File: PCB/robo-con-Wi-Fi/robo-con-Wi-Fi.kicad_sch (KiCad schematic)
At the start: 118 parts, among them J1 Conn_01x04, J2 SMA-J, J3 Conn_01x05, J4 Conn_01x01, J5 Conn_01x02, J6 Conn_01x01, J7 Conn_01x06, Q1 2SC3325-Y, SW1 SW_Push, SW2 SW_Push, U1 STM32H723VGTx, U10 MCP73831-2-OT, U11 LM66100DCK, U12 NJM12877, U13 TXB0606DYYR, U14 TPS628513DRLR, U15 LM66100DCK, U18 USB_Type-C, U2 LBEE5HY2FY, U3 TXU0204, U5 RKJXV122400R, U6 IS25LP064D-JLLE, U7 RKJXV122400R, U8 TMHU28, U9 TMHU28, Y2 XRCGB25M000FFS1AR0

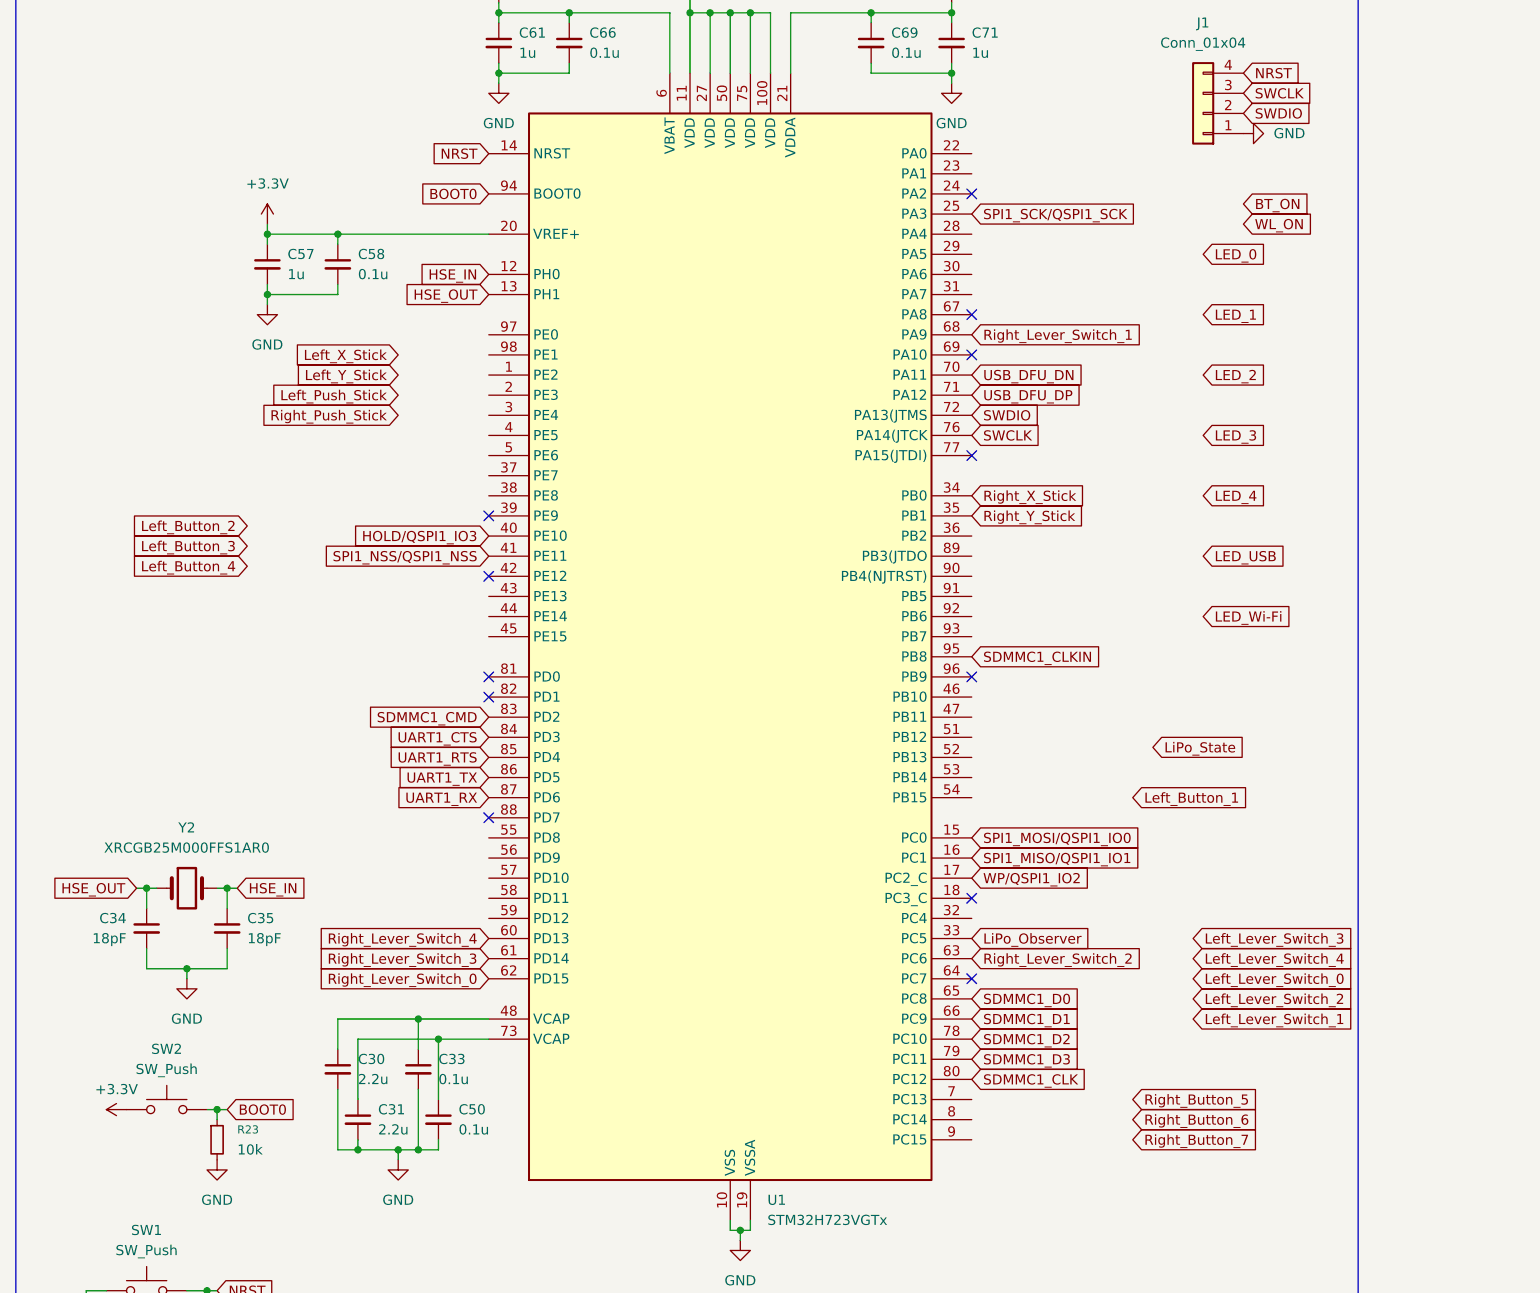
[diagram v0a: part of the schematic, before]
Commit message: PCB配線した　長さ合わせた後確認
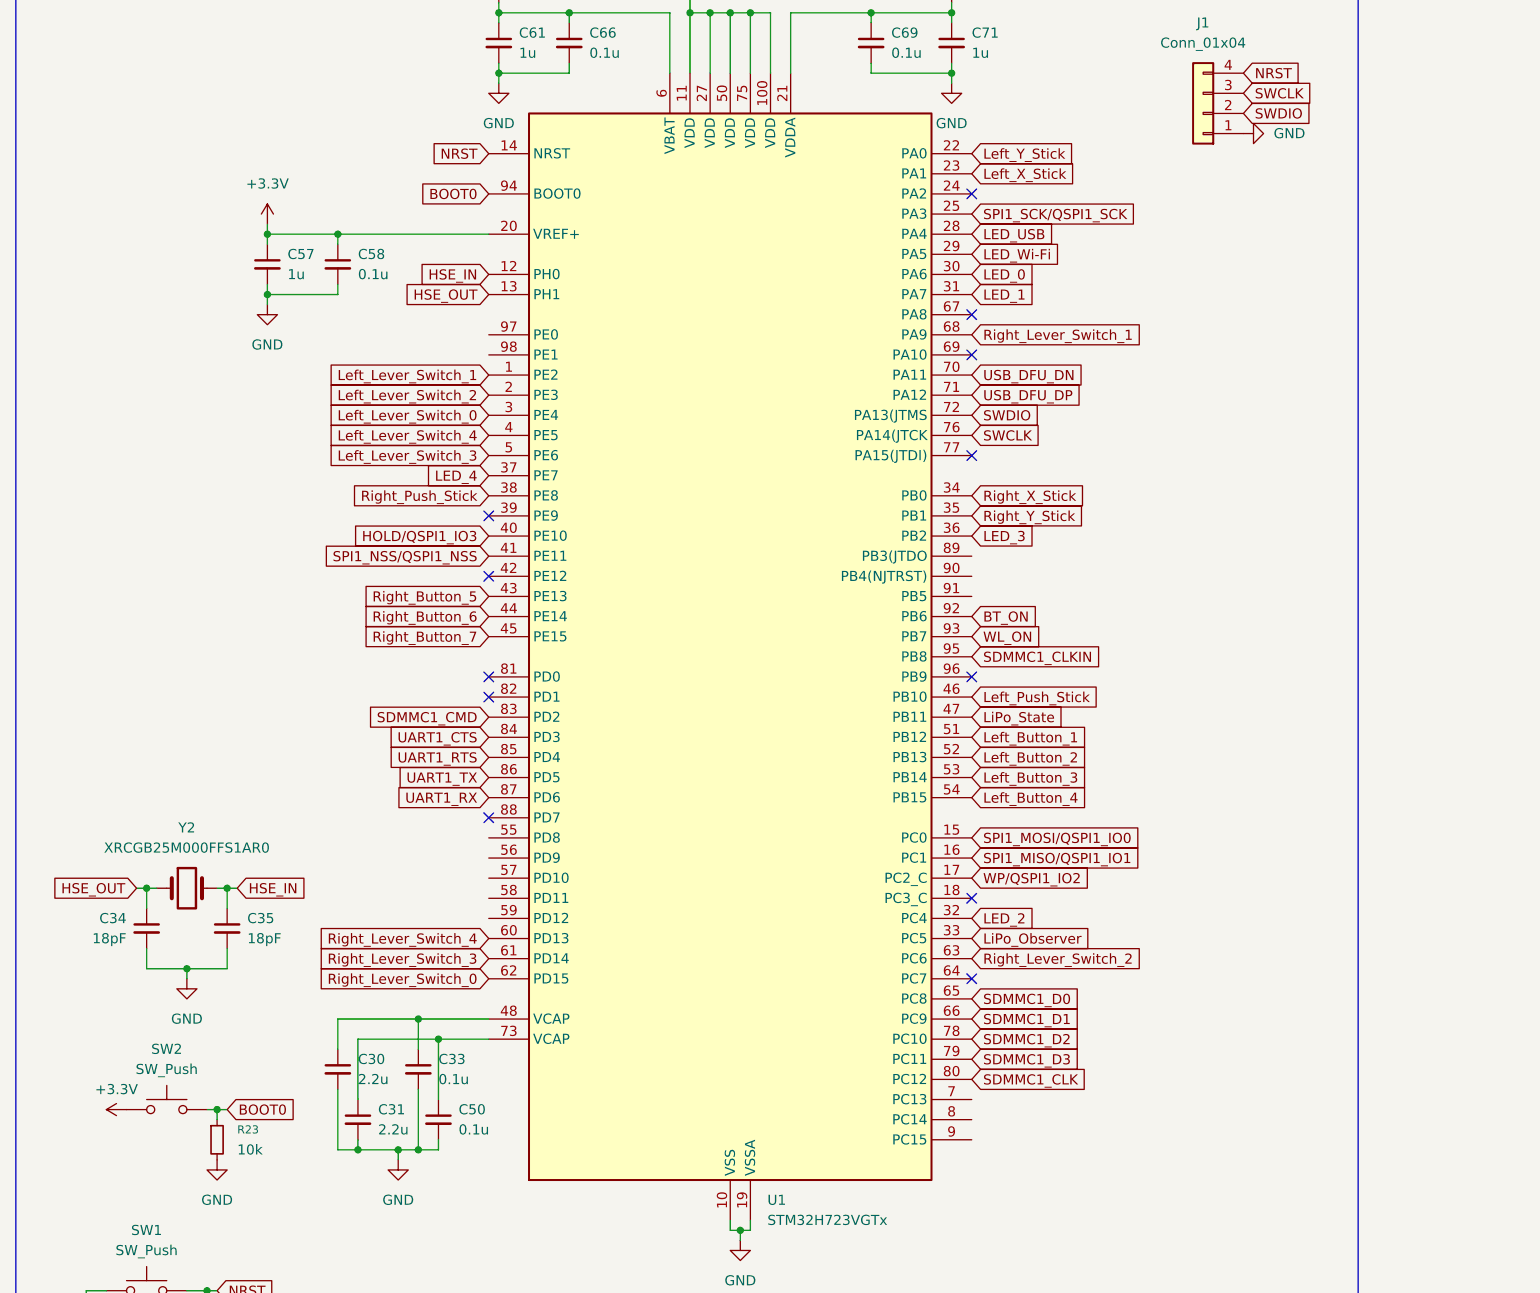
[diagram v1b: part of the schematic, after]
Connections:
- net BT_ON: now also U1.92 (PB6)
- net LED_0: now also U1.30 (PA6)
- net LED_1: now also U1.31 (PA7)
- net LED_2: now also U1.32 (PC4)
- net LED_3: now also U1.36 (PB2)
- net LED_4: now also U1.37 (PE7)
- net LED_USB: now also U1.28 (PA4)
- net LED_Wi-Fi: now also U1.29 (PA5)
- net Left_Button_1: now also U1.51 (PB12)
- net Left_Button_2: now also U1.52 (PB13)
- net Left_Button_3: now also U1.53 (PB14)
- net Left_Button_4: now also U1.54 (PB15)
- net Left_Lever_Switch_0: now also U1.3 (PE4)
- net Left_Lever_Switch_1: now also U1.1 (PE2)
- net Left_Lever_Switch_2: now also U1.2 (PE3)
- net Left_Lever_Switch_3: now also U1.5 (PE6)
- net Left_Lever_Switch_4: now also U1.4 (PE5)
- net Left_Push_Stick: now also U1.46 (PB10)
- net Left_X_Stick: now also U1.23 (PA1)
- net Left_Y_Stick: now also U1.22 (PA0)
- net LiPo_State: now also U1.47 (PB11)
- net Right_Button_5: now also U1.43 (PE13)
- net Right_Button_6: now also U1.44 (PE14)
- net Right_Button_7: now also U1.45 (PE15)
- net Right_Push_Stick: now also U1.38 (PE8)
- net WL_ON: now also U1.93 (PB7)
